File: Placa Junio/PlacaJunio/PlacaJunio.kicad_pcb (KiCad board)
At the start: 2 copper layers, 32 x 110 mm, 24 parts, among them IC1 LC86LICMD, J3 Terminal P2, J4 Terminal P1, J5 Terminal P3, J6 Terminal P4, Q2 IRLML0030, Q3 IRLML0030, Q4 IRLML0030, U5 TSR2-2433N

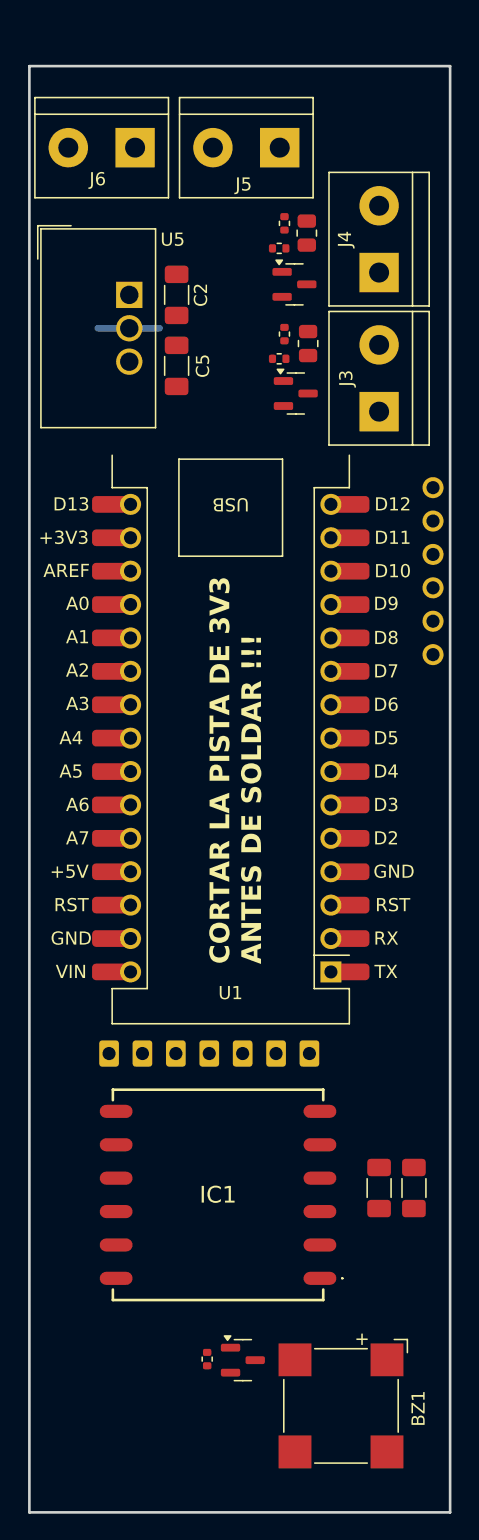
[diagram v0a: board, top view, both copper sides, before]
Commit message: Version 1
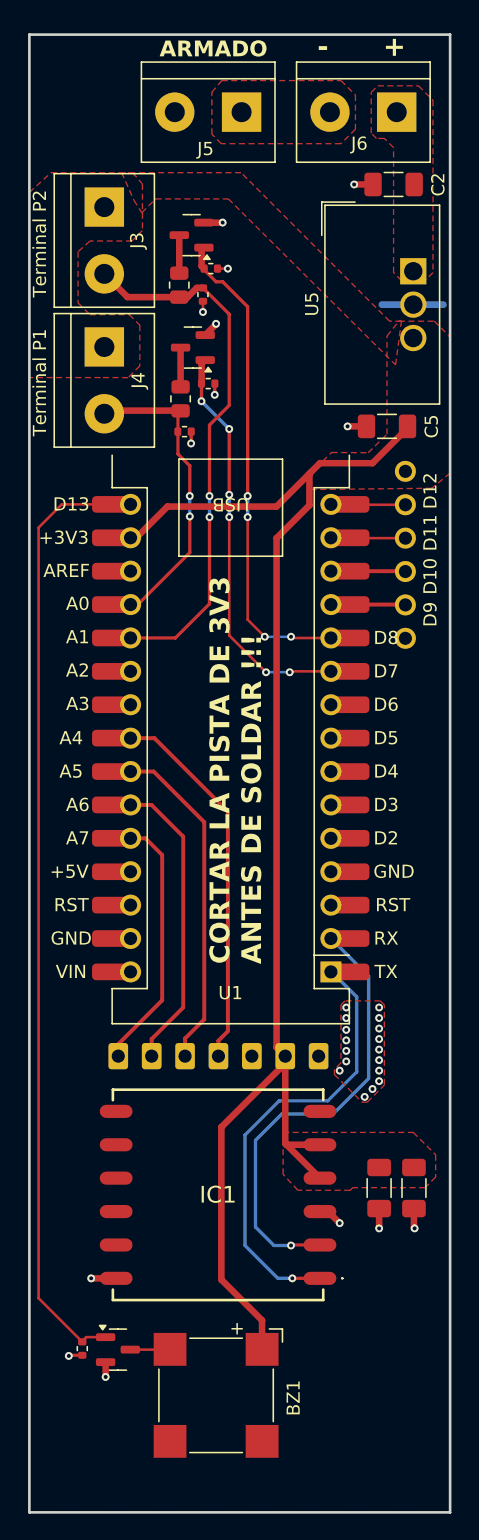
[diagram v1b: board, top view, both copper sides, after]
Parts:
- moved J3 26.1 mm to (136.5, 45.4), turned to -90 degrees
- moved U5 21.7 mm to (160.0, 50.3)
- moved J4 21.7 mm to (136.5, 56.1), turned to -90 degrees
- moved J6 20.1 mm to (158.7, 38.2)
- moved C2 18.5 mm to (158.5, 43.7), turned to 180 degrees
- moved R15 17.6 mm to (142.6, 62.5), turned to 0 degrees
- moved C5 16.6 mm to (158.0, 62.1), turned to 180 degrees
- moved R14 15.8 mm to (142.3, 60.0), turned to 90 degrees
- moved Q2 14.4 mm to (143.1, 47.6), turned to 180 degrees
- moved R7 11.6 mm to (144.4, 58.8), turned to 0 degrees
- moved R17 10.8 mm to (142.2, 51.4), turned to 90 degrees
- moved Q4 9.53 mm to (137.5, 132.3)
- moved R9 9.53 mm to (134.8, 132.2)
- moved BZ1 9.53 mm to (145.0, 135.8)
- moved Q3 9.10 mm to (143.2, 56.1), turned to 180 degrees
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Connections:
- J5 pad 1: GND -> Net-(J5-Pin_1)
- J5 pad 2: Net-(J5-Pin_2) -> GND
- J6 pad 1: Net-(J5-Pin_2) -> +BATT
- J6 pad 2: +BATT -> Net-(J5-Pin_1)
- U1 pad 1: unconnected-(U1-D_13-Pad1) -> /Buzzer
- U1 pad 10: unconnected-(U1-A6-Pad10)_1 -> /M1_LoRa
- U1 pad 11: unconnected-(U1-A7-Pad11)_1 -> /M0_LoRa
- U1 pad 20: /TX_LoRa -> unconnected-(U1-D2-Pad20)
- U1 pad 21: /RX_LoRa -> unconnected-(U1-D3-Pad21)_1
- U1 pad 22: /M1_LoRa -> unconnected-(U1-D4-Pad22)
- U1 pad 23: /M0_LoRa -> unconnected-(U1-D5-Pad23)_1
- U1 pad 24: /Buzzer -> unconnected-(U1-D6-Pad24)
- U1 pad 25: unconnected-(U1-D7-Pad25) -> /PARACAIDAS 1
- U1 pad 26: unconnected-(U1-D8-Pad26) -> /PARACAIDAS 2
- U1 pad 4: unconnected-(U1-A0-Pad4) -> /SENSE 1
- U1 pad 5: /SENSE 1 -> /SENSE 2
- U1 pad 6: /PARACAIDAS 1 -> unconnected-(U1-A2-Pad6)_1
- U1 pad 7: /SENSE 2 -> unconnected-(U1-A3-Pad7)_1
- U1 pad 8: /PARACAIDAS 2 -> /TX_LoRa
- U1 pad 9: unconnected-(U1-A5-Pad9) -> /RX_LoRa
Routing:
- net +3V3: track 0.00 -> 108.8 mm
- net /Buzzer: track 0.00 -> 73.0 mm
- net /SENSE 2: track 0.00 -> 41.3 mm, vias 0 -> 2
- net /PARACAIDAS 2: track 0.00 -> 37.0 mm, vias 0 -> 4
- net /TX_GPS: track 0.00 -> 34.5 mm, vias 0 -> 1
- net /RX_GPS: track 0.00 -> 34.1 mm, vias 0 -> 1
- net /PARACAIDAS 1: track 0.00 -> 31.3 mm, vias 0 -> 6
- net /TX_LoRa: track 0.00 -> 28.6 mm
- net /RX_LoRa: track 0.00 -> 25.6 mm
- net /SENSE 1: track 0.00 -> 23.0 mm, vias 0 -> 2
- net /M1_LoRa: track 0.00 -> 22.7 mm
- net /M0_LoRa: track 0.00 -> 19.6 mm
- net GND: track 4.70 -> 22.5 mm, vias 0 -> 31
- net /SD_CS: track 0.00 -> 6.28 mm
- net /SCK: track 0.00 -> 6.28 mm
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- added copper zone on F.Cu, net +3V3
- added copper zone on F.Cu, net +BATT
- added copper zone on F.Cu, net GND
- added copper zone on F.Cu, net Net-(J5-Pin_1)
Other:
- board size 32 x 110 mm -> 32 x 112.4 mm
- board text added: "+"
- board text added: "-"
- board text added: "ARMADO"
